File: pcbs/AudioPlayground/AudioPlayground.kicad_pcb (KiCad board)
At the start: 6 copper layers, 69.7 x 22.9 mm, 144 parts, among them J1 Conn_01x07_Socket, J2 Conn_Battery, J3 USB_C_Receptacle_USB2.0_14P, J4 TC2030, J5 Conn_01x12_Pin, J7 Conn_01x16_Pin, J9 Conn_01x07_Socket, U1 nRF5340-QKxx, U10 MCP73831-2-OT, U11 SN74LVC1G66DRYR, U12 AP2280, U13 SN74LVC1G66DRYR, U14 TS3USB221ARSER, U15 USBLC6-2P6, U16 SN74LVC1G66DRYR, U17 SN74LVC1G66DRYR, U19 GTD3526BA-1N, U2 R7FA4M2AB3CNE, U20 GTD3526BA-1N, U21 SN74LVC1G66DRYR, U3 USB2422/MJ, U4 MAX9867, U5 XC6209F332MR, U6 XC6209F182MR, U7 DMM-4326-T-R, U8 DMM-4326-T-R, U9 LM66200DRLR, Y1 32MHz, Y2 12mHz, Y3 24MHz, Y4 32.768kHz

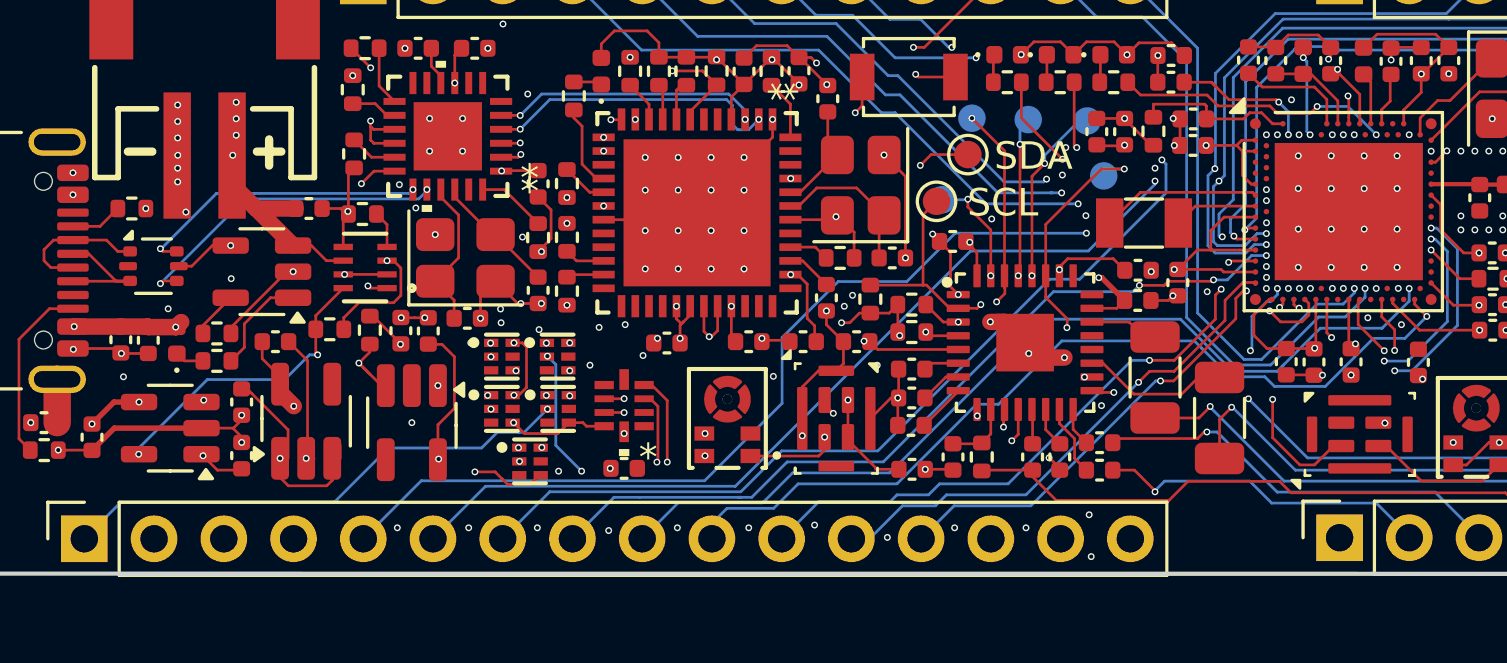
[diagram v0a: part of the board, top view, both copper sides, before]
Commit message: Cleanup
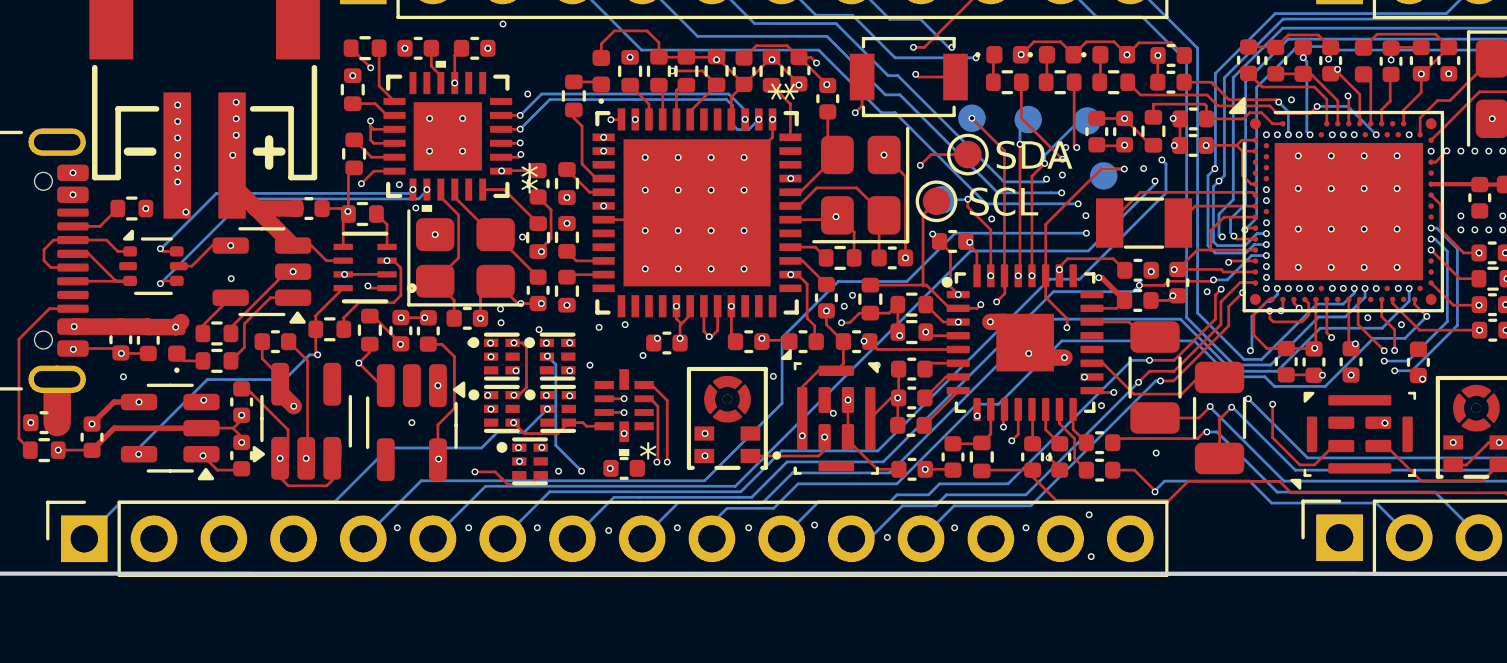
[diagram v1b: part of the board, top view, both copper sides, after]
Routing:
- net /IO/WING_EN: track 18.5 -> 18.0 mm
- net VBUS: vias 7 -> 6
- net GND: vias 245 -> 246
